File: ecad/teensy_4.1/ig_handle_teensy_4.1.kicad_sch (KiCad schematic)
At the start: 1 part, among them U1 Teensy 4.1

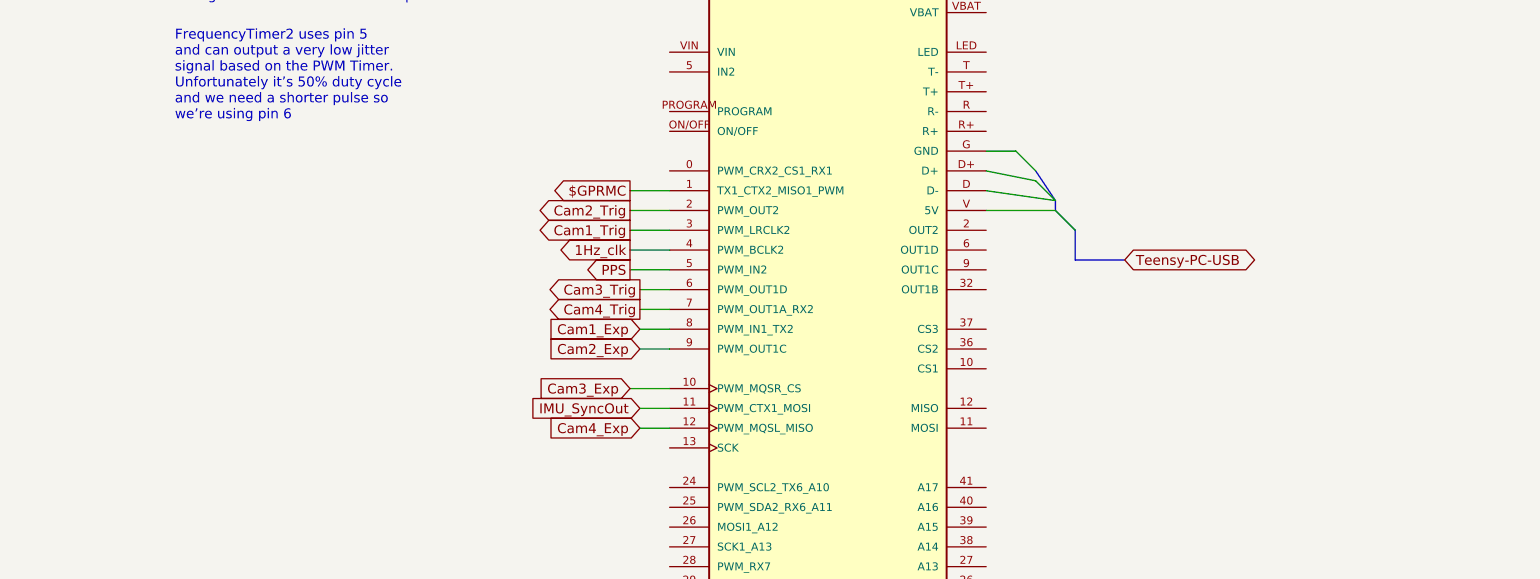
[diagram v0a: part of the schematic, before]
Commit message: Update eCad Files
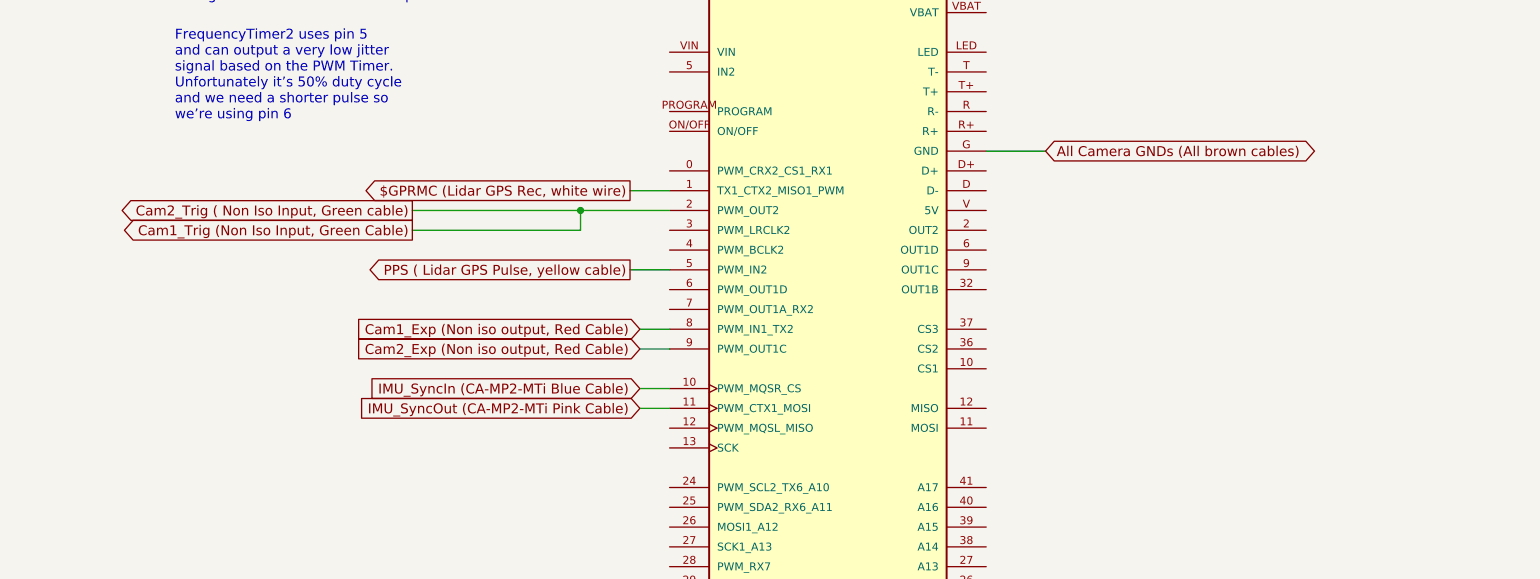
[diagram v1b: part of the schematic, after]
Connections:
- net Cam2_Exp is gone; now on net Cam2_Exp (Non iso output, Red Cable): U1.9 (PWM_OUT1C)
- net Cam2_Trig is gone; now on net Cam1_Trig (Non Iso Input, Green Cable): U1.2 (PWM_OUT2)
- net Cam3_Exp is gone; now on net IMU_SyncIn (CA-MP2-MTi Blue Cable): U1.10 (PWM_MQSR_CS)
- net IMU_SyncOut is gone; now on net IMU_SyncOut (CA-MP2-MTi Pink Cable): U1.11 (PWM_CTX1_MOSI)
- net PPS is gone; now on net PPS ( Lidar GPS Pulse, yellow cable): U1.5 (PWM_IN2)
- net IMU_SyncIn (CA-MP2-MTi Blue Cable): now reaches U1.10 (PWM_MQSR_CS)
- net IMU_SyncOut (CA-MP2-MTi Pink Cable): now reaches U1.11 (PWM_CTX1_MOSI)
- net Cam1_Trig (Non Iso Input, Green Cable): now reaches U1.2 (PWM_OUT2)
- net PPS ( Lidar GPS Pulse, yellow cable): now reaches U1.5 (PWM_IN2)
- net Cam2_Exp (Non iso output, Red Cable): now reaches U1.9 (PWM_OUT1C)
- net All Camera GNDs (All brown cables): now reaches U1.G (GND)
- net $GPRMC renamed $GPRMC (Lidar GPS Rec, white wire)
- net 1Hz_clk: no longer names the net of U1.4 (PWM_BCLK2)
- net Cam1_Exp renamed Cam1_Exp (Non iso output, Red Cable)
- net Cam1_Trig: no longer names the net of U1.3 (PWM_LRCLK2)
- removed net Cam3_Trig: U1.6 (PWM_OUT1D)
- removed net Cam4_Exp: U1.12 (PWM_MQSL_MISO)
- net Cam4_Trig: no longer names the net of U1.7 (PWM_OUT1A_RX2)
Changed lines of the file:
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@@
 (kicad_sch (version 20211123) (generator eeschema)
   (paper "A4")
-  (bus_entry (at 140.97 78.74) (size 2.54 2.54)
-    (stroke (width 0) (type default) (color 0 0 0 0))
-  )
-  (bus_entry (at 135.89 71.12) (size 2.54 2.54)
-    (stroke (width 0) (type default) (color 0 0 0 0))
-  )
-  (bus_entry (at 138.43 74.93) (size 2.54 2.54)
-    (stroke (width 0) (type default) (color 0 0 0 0))
-  )
-  (wire (pts (xy 91.44 91.44) (xy 87.63 91.44))
-    (stroke (width 0) (type default) (color 0 0 0 0))
-  )
-  (wire (pts (xy 135.89 71.12) (xy 132.08 71.12))
-    (stroke (width 0) (type default) (color 0 0 0 0))
-  )
-  (wire (pts (xy 140.97 77.47) (xy 132.08 76.2))
-    (stroke (width 0) (type default) (color 0 0 0 0))
+  (junction (at 80.01 78.74) (diameter 0) (color 0 0 0 0)
   )
   (wire (pts (xy 91.44 86.36) (xy 86.36 86.36))
@@
     (stroke (width 0) (type default) (color 0 0 0 0))
   )
-  (bus (pts (xy 140.97 78.74) (xy 143.51 81.28))
-    (stroke (width 0) (type default) (color 0 0 0 0))
-  )
-  (wire (pts (xy 86.36 83.82) (xy 91.44 83.82))
-    (stroke (width 0) (type default) (color 0 0 0 0))
-  )
-  (wire (pts (xy 86.36 81.28) (xy 91.44 81.28))
-    (stroke (width 0) (type default) (color 0 0 0 0))
-  )
-  (wire (pts (xy 86.36 101.6) (xy 91.44 101.6))
-    (stroke (width 0) (type default) (color 0 0 0 0))
-  )
-  (wire (pts (xy 138.43 74.93) (xy 132.08 73.66))
+  (wire (pts (xy 58.42 81.28) (xy 80.01 81.28))
     (stroke (width 0) (type default) (color 0 0 0 0))
   )
@@
     (stroke (width 0) (type default) (color 0 0 0 0))
   )
-  (wire (pts (xy 87.63 88.9) (xy 91.44 88.9))
+  (wire (pts (xy 132.08 71.12) (xy 139.7 71.12))
     (stroke (width 0) (type default) (color 0 0 0 0))
   )
-  (bus (pts (xy 140.97 77.47) (xy 140.97 78.74))
+  (wire (pts (xy 87.63 101.6) (xy 91.44 101.6))
     (stroke (width 0) (type default) (color 0 0 0 0))
   )
-  (bus (pts (xy 143.51 85.09) (xy 149.86 85.09))
+  (wire (pts (xy 58.42 78.74) (xy 80.01 78.74))
     (stroke (width 0) (type default) (color 0 0 0 0))
   )
-  (bus (pts (xy 138.43 73.66) (xy 140.97 77.47))
+  (wire (pts (xy 80.01 78.74) (xy 91.44 78.74))
     (stroke (width 0) (type default) (color 0 0 0 0))
   )
-  (wire (pts (xy 132.08 78.74) (xy 140.97 78.74))
-    (stroke (width 0) (type default) (color 0 0 0 0))
-  )
-  (wire (pts (xy 86.36 78.74) (xy 91.44 78.74))
+  (wire (pts (xy 80.01 81.28) (xy 80.01 78.74))
     (stroke (width 0) (type default) (color 0 0 0 0))
   )
@@
     (stroke (width 0) (type default) (color 0 0 0 0))
   )
-  (wire (pts (xy 87.63 106.68) (xy 91.44 106.68))
-    (stroke (width 0) (type default) (color 0 0 0 0))
-  )
   (wire (pts (xy 91.44 104.14) (xy 87.63 104.14))
     (stroke (width 0) (type default) (color 0 0 0 0))
   )
-  (bus (pts (xy 143.51 81.28) (xy 143.51 85.09))
-    (stroke (width 0) (type default) (color 0 0 0 0))
-  )
   (image (at 251.46 124.46) (scale 1.1768)
     (data
@@
     (effects (font (size 1.4986 1.4986)) (justify left bottom))
   )
-  (global_label "IMU_SyncOut" (shape input) (at 87.63 104.14 180) (fields_autoplaced)
-    (effects (font (size 1.27 1.27)) (justify right))
-    (property "Intersheet References" "${INTERSHEET_REFS}" (id 0) (at 6.35 29.21 0)
-      (effects (font (size 1.27 1.27)) hide)
-    )
-  )
-  (global_label "Cam4_Exp" (shape input) (at 87.63 106.68 180) (fields_autoplaced)
+  (global_label "IMU_SyncOut (CA-MP2-MTi Pink Cable)" (shape input) (at 87.63 104.14 180) (fields_autoplaced)
     (effects (font (size 1.27 1.27)) (justify right))
-    (property "Intersheet References" "${INTERSHEET_REFS}" (id 0) (at 6.35 26.67 0)
-      (effects (font (size 1.27 1.27)) hide)
+    (property "Intersheet References" "${INTERSHEET_REFS}" (id 0) (at 46.8145 104.0606 0)
+      (effects (font (size 1.27 1.27)) (justify right) hide)
     )
   )
-  (global_label "Cam3_Exp" (shape input) (at 86.36 101.6 180) (fields_autoplaced)
-    (effects (font (size 1.27 1.27)) (justify right))
-    (property "Intersheet References" "${INTERSHEET_REFS}" (id 0) (at 5.08 29.21 0)
-      (effects (font (size 1.27 1.27)) hide)
-    )
-  )
-  (global_label "Teensy-PC-USB" (shape bidirectional) (at 149.86 85.09 0) (fields_autoplaced)
+  (global_label "All Camera GNDs (All brown cables)" (shape bidirectional) (at 139.7 71.12 0) (fields_autoplaced)
     (effects (font (size 1.27 1.27)) (justify left))
-    (property "Intersheet References" "${INTERSHEET_REFS}" (id 0) (at -2.54 -34.29 0)
-      (effects (font (size 1.27 1.27)) hide)
-    )
-  )
-  (global_label "Cam2_Exp" (shape input) (at 87.63 96.52 180) (fields_autoplaced)
-    (effects (font (size 1.27 1.27)) (justify right))
-    (property "Intersheet References" "${INTERSHEET_REFS}" (id 0) (at 6.35 26.67 0)
-      (effects (font (size 1.27 1.27)) hide)
-    )
-  )
-  (global_label "1Hz_clk" (shape output) (at 86.36 83.82 180) (fields_autoplaced)
-    (effects (font (size 1.27 1.27)) (justify right))
-    (property "Intersheet References" "${INTERSHEET_REFS}" (id 0) (at 6.35 26.67 0)
-      (effects (font (size 1.27 1.27)) hide)
+    (property "Intersheet References" "${INTERSHEET_REFS}" (id 0) (at 177.2498 71.0406 0)
+      (effects (font (size 1.27 1.27)) (justify left) hide)
     )
   )
-  (global_label "Cam3_Trig" (shape output) (at 87.63 88.9 180) (fields_autoplaced)
+  (global_label "Cam2_Exp (Non iso output, Red Cable)" (shape input) (at 87.63 96.52 180) (fields_autoplaced)
     (effects (font (size 1.27 1.27)) (justify right))
-    (property "Intersheet References" "${INTERSHEET_REFS}" (id 0) (at 6.35 26.67 0)
-      (effects (font (size 1.27 1.27)) hide)
+    (property "Intersheet References" "${INTERSHEET_REFS}" (id 0) (at 47.1774 96.4406 0)
+      (effects (font (size 1.27 1.27)) (justify right) hide)
     )
   )
-  (global_label "Cam4_Trig" (shape output) (at 87.63 91.44 180) (fields_autoplaced)
+  (global_label "Cam2_Trig ( Non Iso Input, Green cable)" (shape output) (at 58.42 78.74 180) (fields_autoplaced)
     (effects (font (size 1.27 1.27)) (justify right))
-    (property "Intersheet References" "${INTERSHEET_REFS}" (id 0) (at 6.35 26.67 0)
-      (effects (font (size 1.27 1.27)) hide)
+    (property "Intersheet References" "${INTERSHEET_REFS}" (id 0) (at 16.395 78.6606 0)
+      (effects (font (size 1.27 1.27)) (justify right) hide)
     )
   )
-  (global_label "Cam2_Trig" (shape output) (at 86.36 78.74 180) (fields_autoplaced)
+  (global_label "PPS ( Lidar GPS Pulse, yellow cable)" (shape output) (at 86.36 86.36 180) (fields_autoplaced)
     (effects (font (size 1.27 1.27)) (justify right))
-    (property "Intersheet References" "${INTERSHEET_REFS}" (id 0) (at 6.35 29.21 0)
-      (effects (font (size 1.27 1.27)) hide)
+    (property "Intersheet References" "${INTERSHEET_REFS}" (id 0) (at 47.4193 86.2806 0)
+      (effects (font (size 1.27 1.27)) (justify right) hide)
     )
   )
-  (global_label "PPS" (shape output) (at 86.36 86.36 180) (fields_autoplaced)
+  (global_label "IMU_SyncIn (CA-MP2-MTi Blue Cable)" (shape input) (at 87.63 101.6 180) (fields_autoplaced)
     (effects (font (size 1.27 1.27)) (justify right))
-    (property "Intersheet References" "${INTERSHEET_REFS}" (id 0) (at 6.35 26.67 0)
-      (effects (font (size 1.27 1.27)) hide)
+    (property "Intersheet References" "${INTERSHEET_REFS}" (id 0) (at 48.145 101.5206 0)
+      (effects (font (size 1.27 1.27)) (justify right) hide)
     )
   )
-  (global_label "$GPRMC" (shape output) (at 86.36 76.2 180) (fields_autoplaced)
+  (global_label "$GPRMC (Lidar GPS Rec, white wire)" (shape output) (at 86.36 76.2 180) (fields_autoplaced)
     (effects (font (size 1.27 1.27)) (justify right))
-    (property "Intersheet References" "${INTERSHEET_REFS}" (id 0) (at 6.35 29.21 0)
-      (effects (font (size 1.27 1.27)) hide)
+    (property "Intersheet References" "${INTERSHEET_REFS}" (id 0) (at 48.4474 76.1206 0)
+      (effects (font (size 1.27 1.27)) (justify right) hide)
     )
   )
-  (global_label "Cam1_Exp" (shape input) (at 87.63 93.98 180) (fields_autoplaced)
+  (global_label "Cam1_Exp (Non iso output, Red Cable)" (shape input) (at 87.63 93.98 180) (fields_autoplaced)
     (effects (font (size 1.27 1.27)) (justify right))
-    (property "Intersheet References" "${INTERSHEET_REFS}" (id 0) (at 6.35 26.67 0)
-      (effects (font (size 1.27 1.27)) hide)
+    (property "Intersheet References" "${INTERSHEET_REFS}" (id 0) (at 47.1774 93.9006 0)
+      (effects (font (size 1.27 1.27)) (justify right) hide)
     )
   )
-  (global_label "Cam1_Trig" (shape output) (at 86.36 81.28 180) (fields_autoplaced)
+  (global_label "Cam1_Trig (Non Iso Input, Green Cable)" (shape output) (at 58.42 81.28 180) (fields_autoplaced)
     (effects (font (size 1.27 1.27)) (justify right))
-    (property "Intersheet References" "${INTERSHEET_REFS}" (id 0) (at 6.35 29.21 0)
-      (effects (font (size 1.27 1.27)) hide)
+    (property "Intersheet References" "${INTERSHEET_REFS}" (id 0) (at 17.1812 81.2006 0)
+      (effects (font (size 1.27 1.27)) (justify right) hide)
     )
   )
